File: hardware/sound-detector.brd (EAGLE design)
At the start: 48.3 x 31.8 mm, 58 parts, among them IC1 LMV324, J1 GATORGATOR_MINI, J2 GATORGATOR_MINI, J3 GATORGATOR_MINI, J4 GATORGATOR_MINI, J5 GATORGATOR_MINI

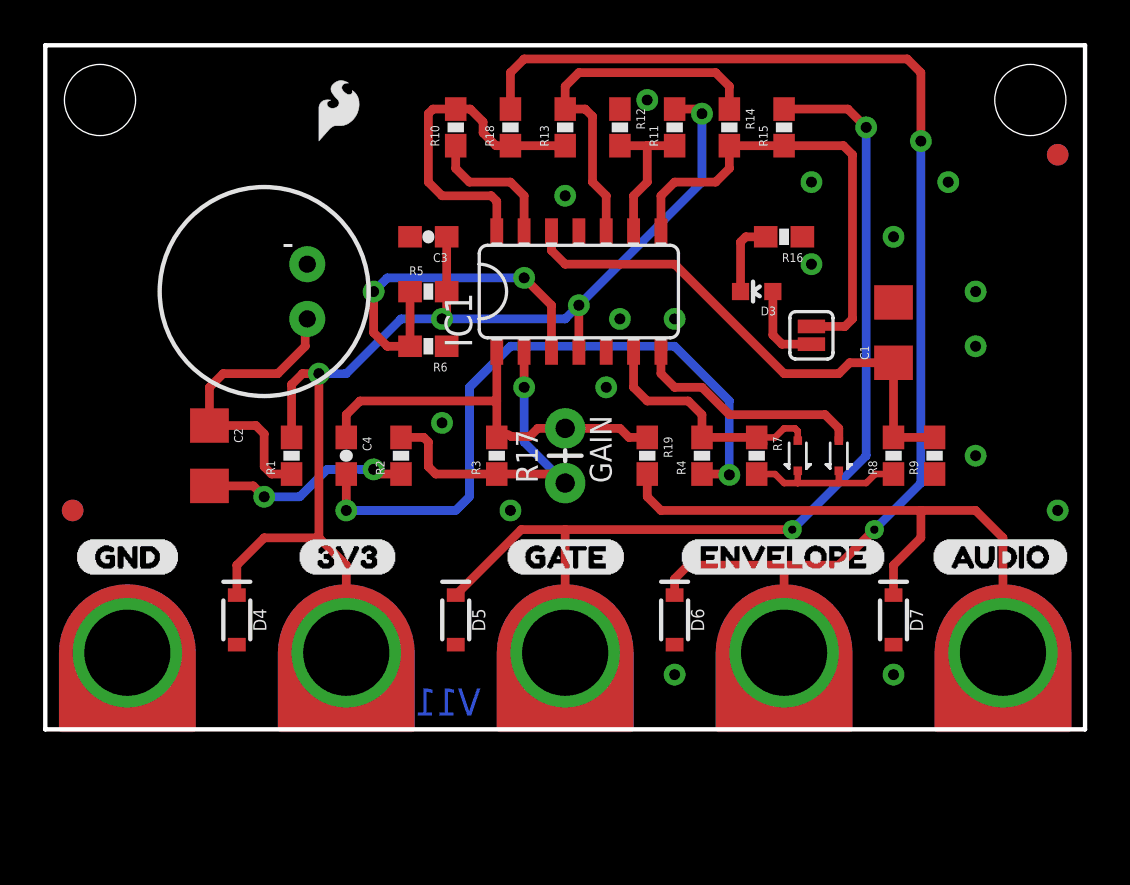
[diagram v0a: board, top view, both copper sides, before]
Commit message: initial layout
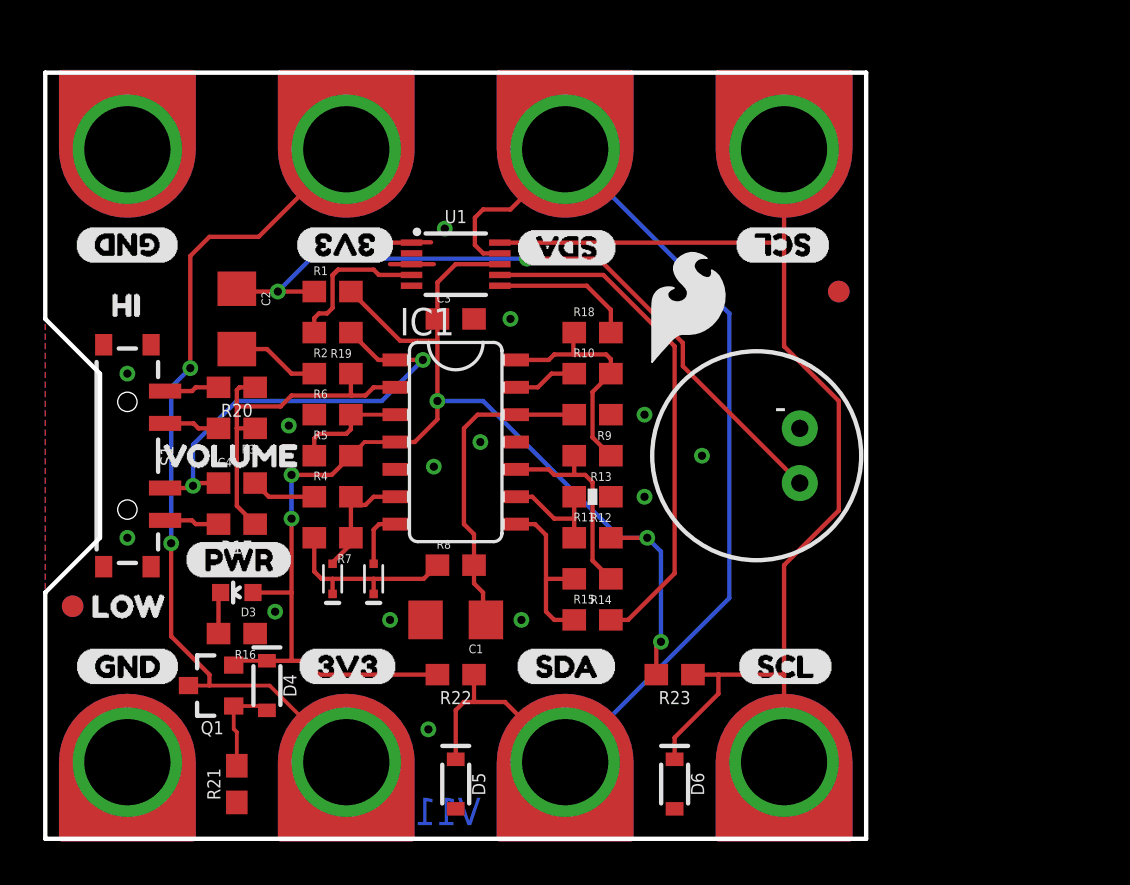
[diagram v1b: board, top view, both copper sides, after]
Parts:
- removed D7: 3.6V, SparkFun-DiscreteSemi:SOD-323
- removed SJ1: Disable LED, SparkFun-Passives:SJ_2S
- removed STANDOFF1, STANDOFF2: STAND-OFF, SparkFun-Electromechanical:STAND-OFF
- added J6, J7, J8: GATORGATOR_MINI, SparkFun-Connectors:GATOR_MINI
- added Q1: 2.5A/30V/105mΩ, SparkFun-DiscreteSemi:SOT23-3
- added R20: 1M, SparkFun-Resistors:0603
- added R21, R22, R23: 10k, SparkFun-Resistors:0603
- added S1: (no value), SparkFun-Switches:SWITCH_SP3T_SMD
- added U$11, U$18: (no value), buzzard_labels (3):3V31
- added U$12, U$19: (no value), buzzard_labels (2):SDA2
- added U$13, U$20: (no value), buzzard_labels (2):SCL1
- added U$14: (no value), buzzard_labels (7):HI0
- added U$15: (no value), buzzard_labels (7):LOW1
- added U$16: (no value), buzzard_labels (7):VOLUME2
- added U$17: (no value), buzzard_labels (2):GND0
- added U1: ADS1015, SparkFun-IC-Conversion:MSOP10
- C1, C2: device SparkFun-Capacitors:1206 -> SparkFun-Capacitors:1206@1
- C3, C4: device SparkFun-Capacitors:0603-CAP -> SparkFun-Capacitors:0603
- D1, D2: value RB751 -> 120mA/40V/370mV
- LOGO1: value OSHW-LOGOM -> OSHW-LOGOS; device SparkFun-Aesthetics:OSHW-LOGO-M -> SparkFun-Aesthetics:OSHW-LOGO-S
- LOGO2: value LOGO-SFENW2 -> SFE_LOGO_NAME_FLAME.2_INCH; device SparkFun-Aesthetics:SFE-NEW-WEB -> SparkFun-Aesthetics:SFE_LOGO_NAME_FLAME_.2
- LOGO3: value LOGO-SFESK -> SFE_LOGO_FLAME.2_INCH; device SparkFun-Aesthetics:SFE-LOGO-FLAME -> SparkFun-Aesthetics:SFE_LOGO_FLAME_.2
- R1, R11, R14, R15, R18, R19, R3, R8: device SparkFun-Resistors:0603-RES -> SparkFun-Resistors:0603
- R10, R13, R2: value 1K -> 1k; device SparkFun-Resistors:0603-RES -> SparkFun-Resistors:0603
- R16: value 2.2k -> 1k; device SparkFun-Resistors:0603-RES -> SparkFun-Resistors:0603
- R17: value GAIN -> 10k; device SparkFun-Resistors:AXIAL-0.1EZ -> SparkFun-Resistors:0603
- R4, R5, R6, R9: value 10K -> 10k; device SparkFun-Resistors:0603-RES -> SparkFun-Resistors:0603
- R7: value 22K -> 22k; device SparkFun-Resistors:0603-RES -> SparkFun-Resistors:0603
- U$10: device buzzard_labels (3):AUDIO4 -> buzzard_labels (2):GND0
- U$2: device buzzard_labels (3):AUDIO4 -> buzzard_labels (2):SCL1
- U$3: device buzzard_labels (3):ENVELOPE3 -> buzzard_labels (2):SDA2
- U$4: device buzzard_labels (3):GATE2 -> buzzard_labels (5):PWR0
- U$8: device buzzard_labels (3):GATE2 -> buzzard_labels (2):SDA2
- U$9: device buzzard_labels (3):ENVELOPE3 -> buzzard_labels (2):SCL1
- moved J1 46.6 mm to (3.81, 31.8), turned to 180 degrees
- moved U$10 44.0 mm to (6.22, 27.6), flipped to the top, turned to 180 degrees
- moved R16 31.4 mm to (8.89, 9.53)
- moved D3 27.9 mm to (8.89, 11.4)
- moved R15 24.5 mm to (25.4, 10.2), turned to 0 degrees
- moved LOGO1 24.4 mm to (19.1, 3.17), turned to 0 degrees
- moved C1 24.3 mm to (19.1, 10.2), turned to 180 degrees
- moved MIC1 24.1 mm to (33.0, 17.8)
- moved D1 22.3 mm to (13.3, 12.1)
- moved D2 22.3 mm to (15.2, 12.1)
- moved R14 21.9 mm to (25.4, 12.1), turned to 180 degrees
- moved R8 20.9 mm to (19.1, 12.7), turned to 0 degrees
- moved R7 20.1 mm to (13.3, 14.0), turned to 180 degrees
- moved R11 19.4 mm to (25.4, 14.0), turned to 0 degrees
- moved LOGO3 18.8 mm to (29.8, 24.6)
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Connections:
- removed net N$12: D3.A, SJ1.1
- new net N$13: R17.2, S1.4
- new net N$14: R3.2, S1.2
- new net N$18: R20.2, S1.1
- new net N$19: J4.P$2, J8.P$2, Q1.3
- new net N$20: D4.A, Q1.1, R21.2
- new net SCL: D6.C, J2.P$2, J7.P$2, R23.1, U1.10
- new net SDA: D5.C, J3.P$2, J6.P$2, R22.1, U1.9
- net 3.3V: now also D3.A, Q1.2, R22.2, R23.2, U1.8; no longer J4.P$2
- net AUDIO: now also U1.4; no longer D7.C, J1.P$2
- net ENVELOPE: now also U1.6; no longer D6.C, J2.P$2
- net GATE: now also U1.7; no longer D5.C, J3.P$2
- net GND: now also J1.P$2, R21.1, U1.1, U1.3; no longer D4.A, D7.A
- net N$: now also S1.3; no longer R17.P$2, R3.2
- net N$17: no longer SJ1.2
- net N$4: now also R17.1, R20.1; no longer R17.P$1
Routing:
- net ENVELOPE: track 59.9 -> 6.67 mm, vias 2 -> 0
- net SDA: track 0.00 -> 53.0 mm
- net SCL: track 0.00 -> 52.8 mm
- net N$19: track 0.00 -> 39.1 mm, vias 0 -> 2
- net N$6: track 31.4 -> 3.01 mm, vias 2 -> 0
- net GATE: track 46.8 -> 23.9 mm, vias 2 -> 0
- net AUDIO: track 28.1 -> 7.47 mm
- net N$1: track 14.0 -> 33.5 mm, vias 0 -> 2
- net N$17: track 22.0 -> 8.35 mm
- net N$2: track 17.6 -> 5.42 mm, vias 2 -> 0
- net N$10: track 24.7 -> 14.7 mm
- net 3.3V: track 55.2 -> 63.4 mm, vias 4 -> 5
- net N$8: track 10.9 -> 2.70 mm
- net N$16: track 17.3 -> 9.54 mm
- net N$7: track 12.1 -> 5.68 mm
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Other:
- board size 48.3 x 31.8 mm -> 38.1 x 35.6 mm
